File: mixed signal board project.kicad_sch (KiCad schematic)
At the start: 0 parts

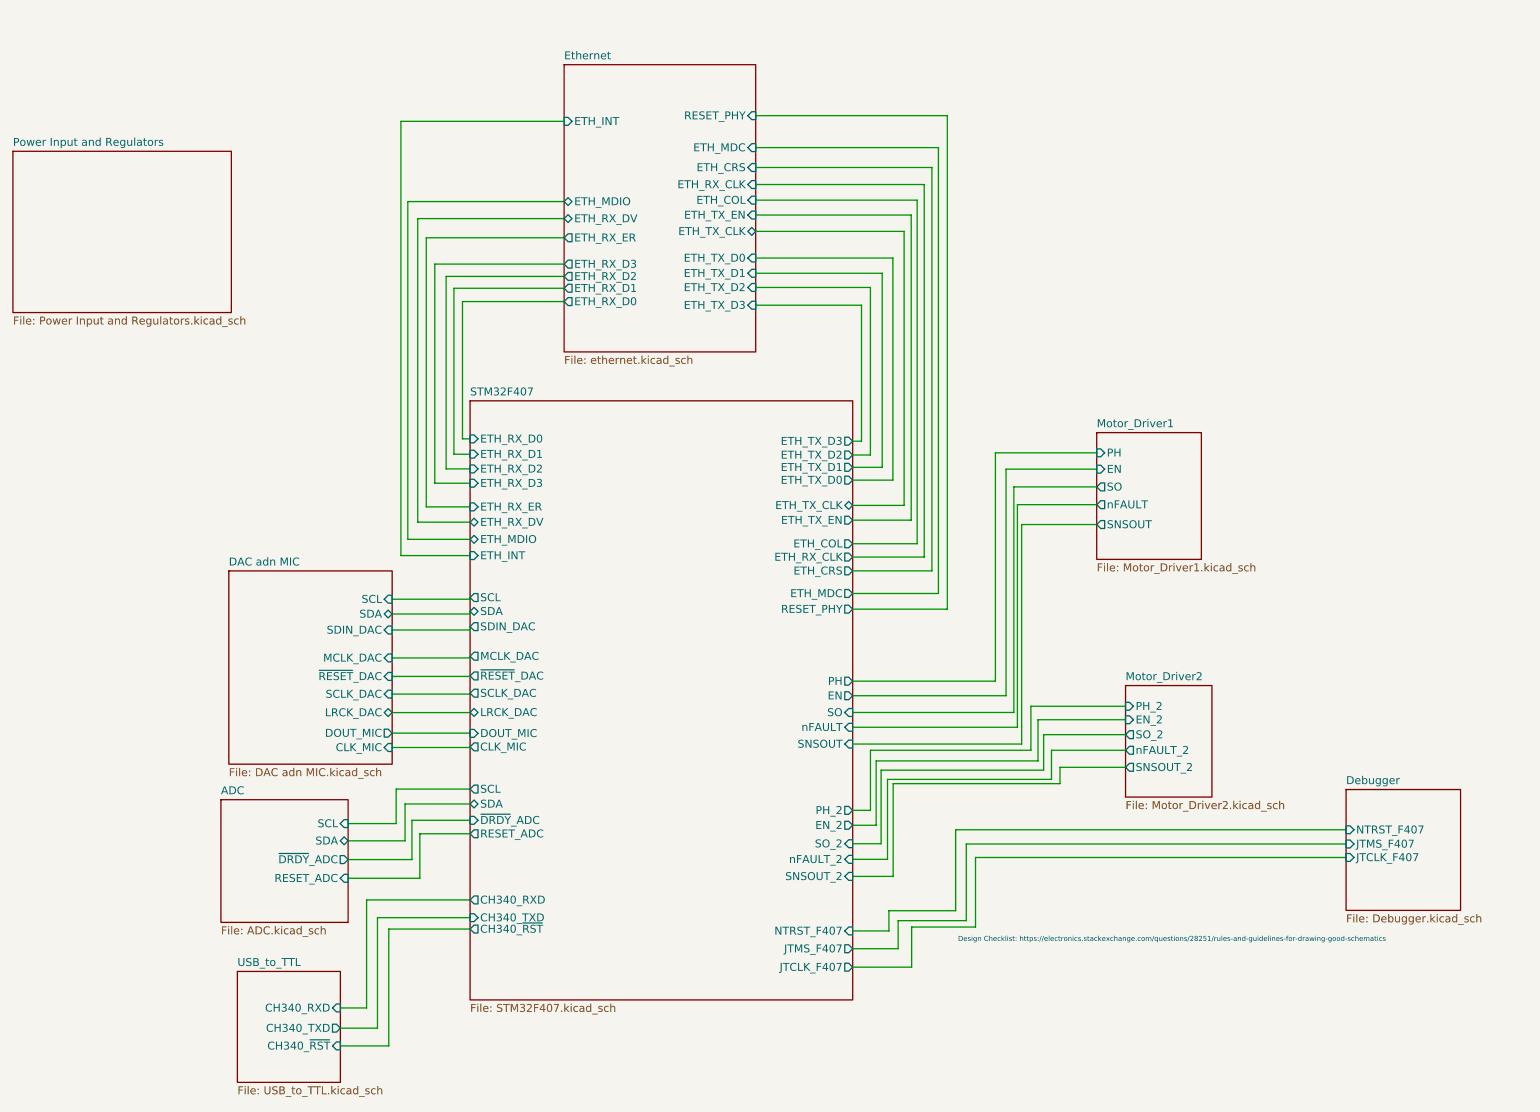
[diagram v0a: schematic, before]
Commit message: some additions
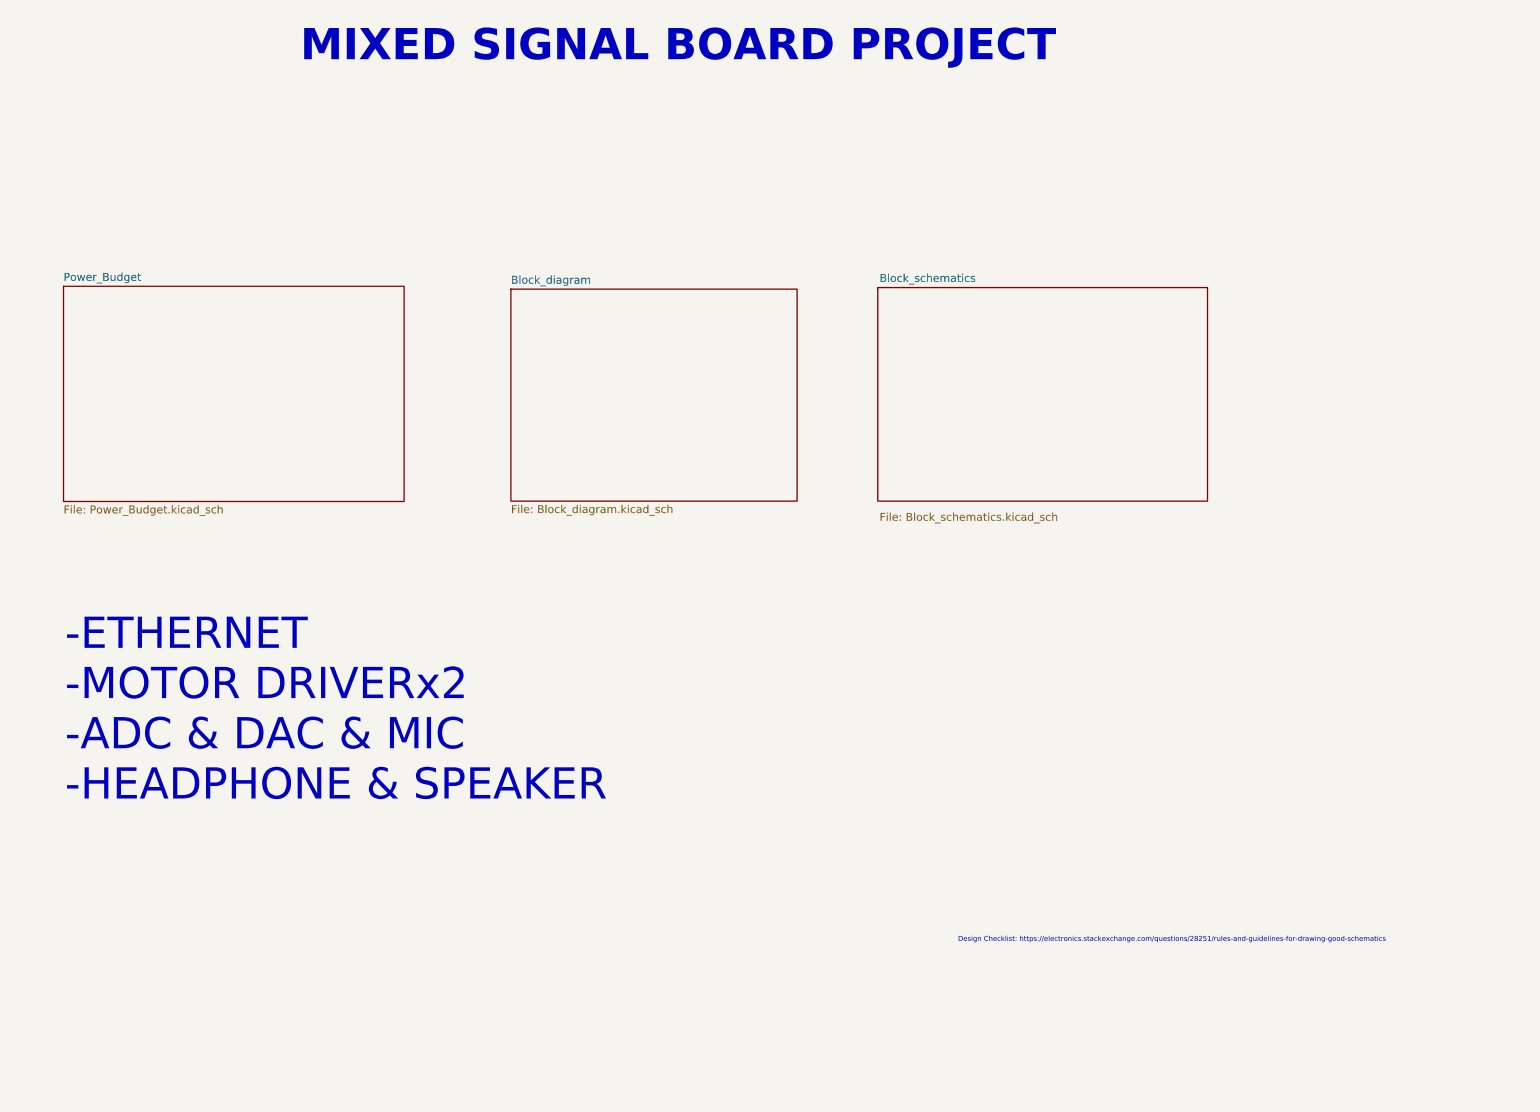
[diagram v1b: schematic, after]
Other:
- removed sheet ADC
- removed sheet DAC adn MIC
- removed sheet Debugger
- removed sheet Ethernet
- removed sheet Motor_Driver1
- removed sheet Motor_Driver2
- removed sheet Power Input and Regulators
- removed sheet STM32F407
- removed sheet USB_to_TTL
- added sheet Block_diagram (Block_diagram.kicad_sch)
- added sheet Block_schematics (Block_schematics.kicad_sch)
- added sheet Power_Budget (Power_Budget.kicad_sch)
- note added: "-ETHERNET -MOTOR DRIVERx2 -ADC & DAC & MIC -HEADPHONE & SPEAKER"
- note added: "MIXED SIGNAL BOARD PROJECT"
